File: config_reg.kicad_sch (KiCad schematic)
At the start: 12 parts, among them U29 74HC377

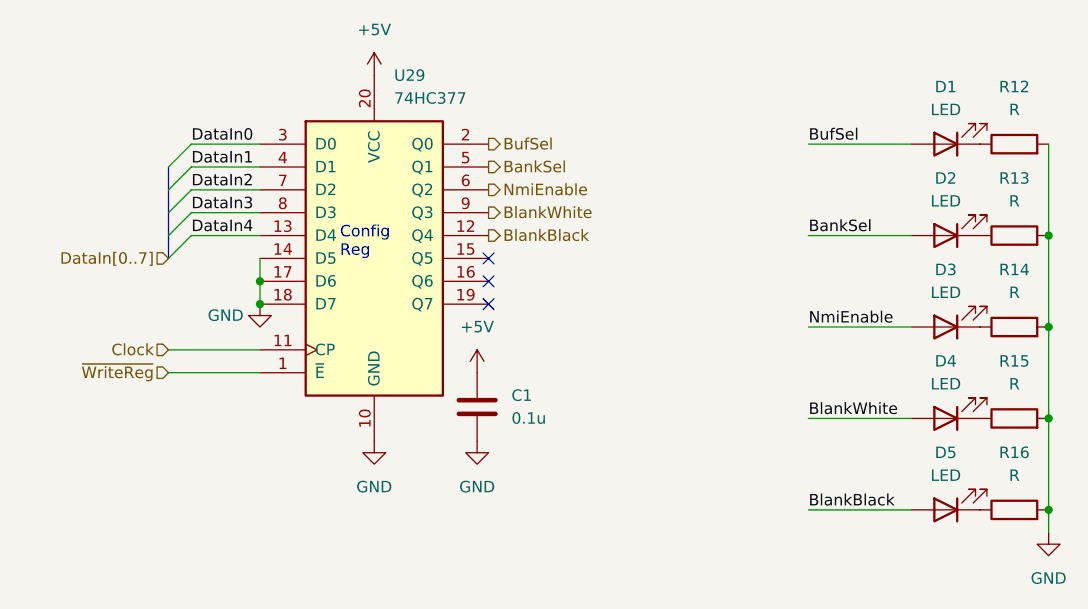
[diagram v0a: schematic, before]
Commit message: Done routing!!
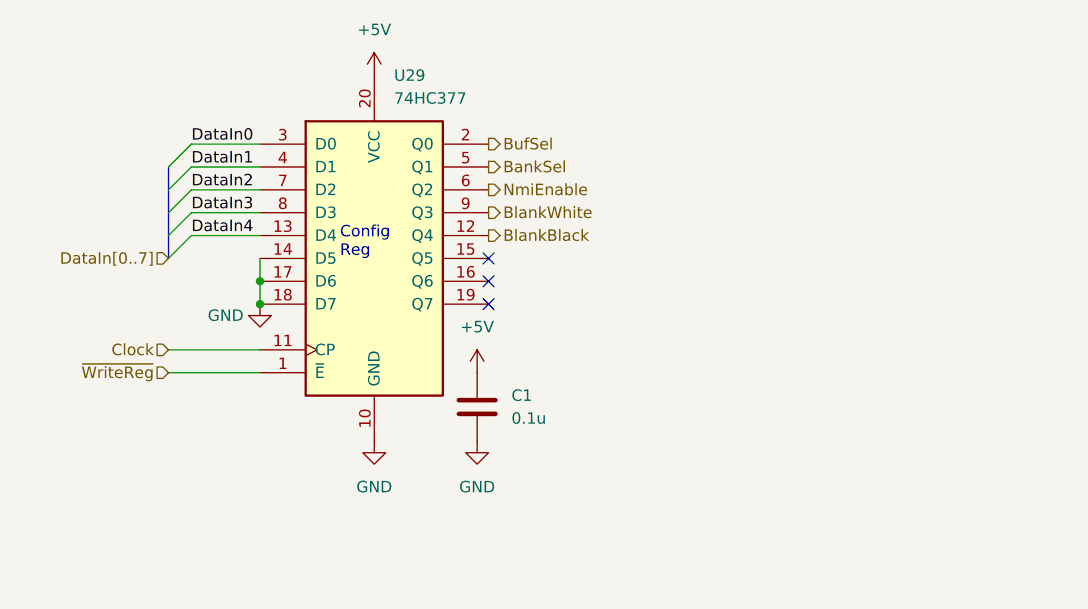
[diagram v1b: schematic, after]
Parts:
- removed D1, D2, D3, D4, D5: LED, symbol Device:LED
- removed R12, R13, R14, R15, R16: R, symbol Device:R
